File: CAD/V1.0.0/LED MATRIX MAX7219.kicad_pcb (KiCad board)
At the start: 2 copper layers, 22 x 54 mm, 92 parts, among them K1 HEADER_MALE_5X1, K2 HEADER_MALE_5X1, U1 MAX7219

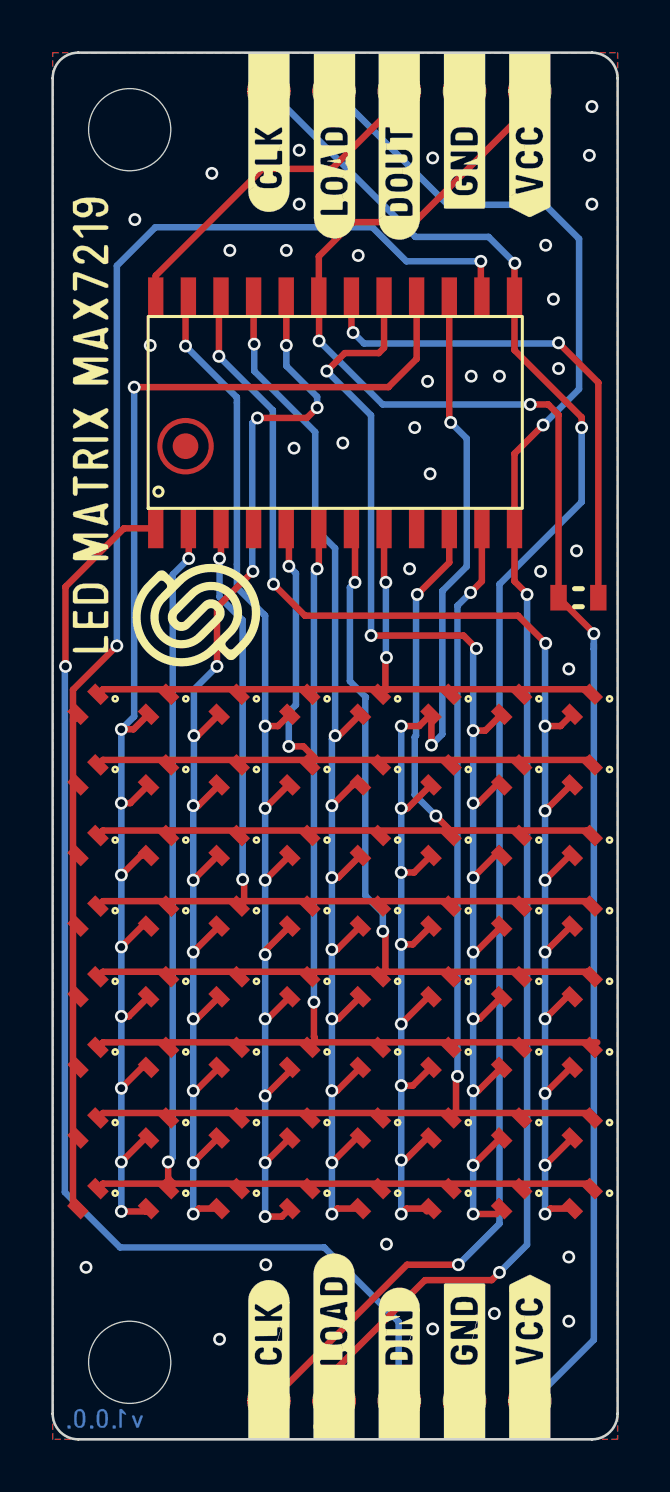
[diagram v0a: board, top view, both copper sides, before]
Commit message: Updating open source files.
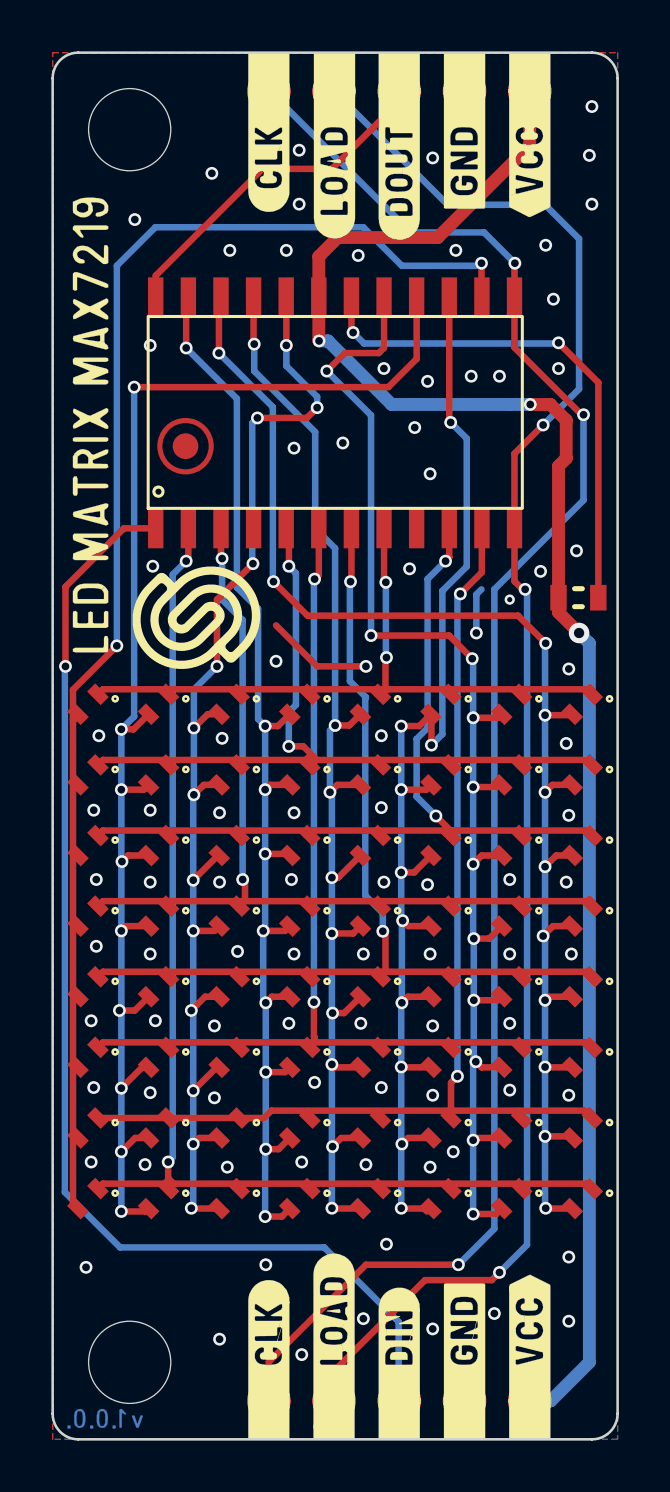
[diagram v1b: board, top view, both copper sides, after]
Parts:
- moved G*** 0.10 mm to (81.0, 120.6)
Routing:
- net GND: track 0.65 -> 6.59 mm, vias 34 -> 91
- net Net-(D15-Pad1): track 53.2 -> 50.8 mm
- net Net-(D16-Pad1): track 57.1 -> 54.8 mm
- net Net-(D12-Pad1): track 47.8 -> 45.7 mm
- net Net-(D14-Pad1): track 50.0 -> 48.2 mm
- net Net-(D13-Pad1): track 48.5 -> 47.0 mm
- net VCC: track 65.3 -> 66.7 mm
- net Net-(D11-Pad1): track 50.1 -> 49.0 mm
- net CLK: track 64.5 -> 65.5 mm
- net Net-(D10-Pad1): track 56.9 -> 56.1 mm
